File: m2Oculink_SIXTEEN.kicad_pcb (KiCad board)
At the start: 2 copper layers, 31.5 x 71.2 mm, 2 parts

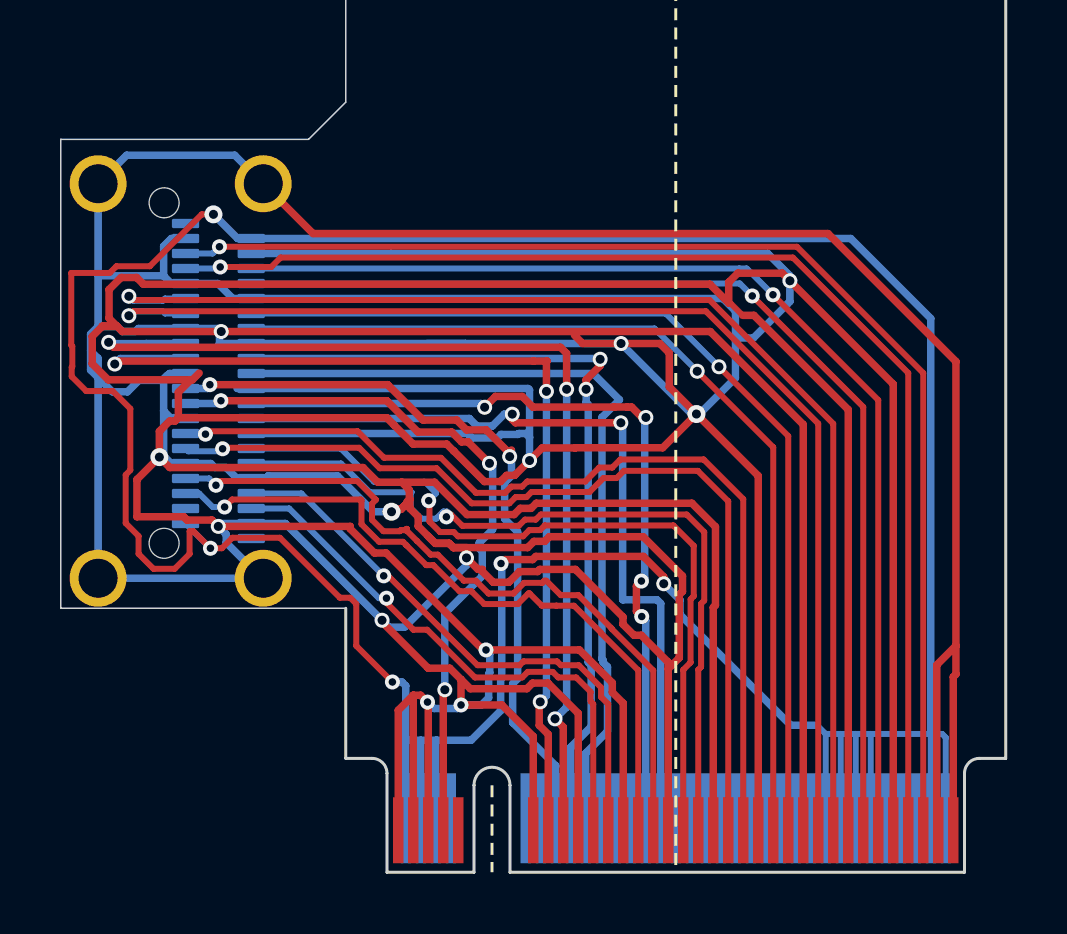
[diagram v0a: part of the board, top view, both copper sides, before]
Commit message: Update PCB
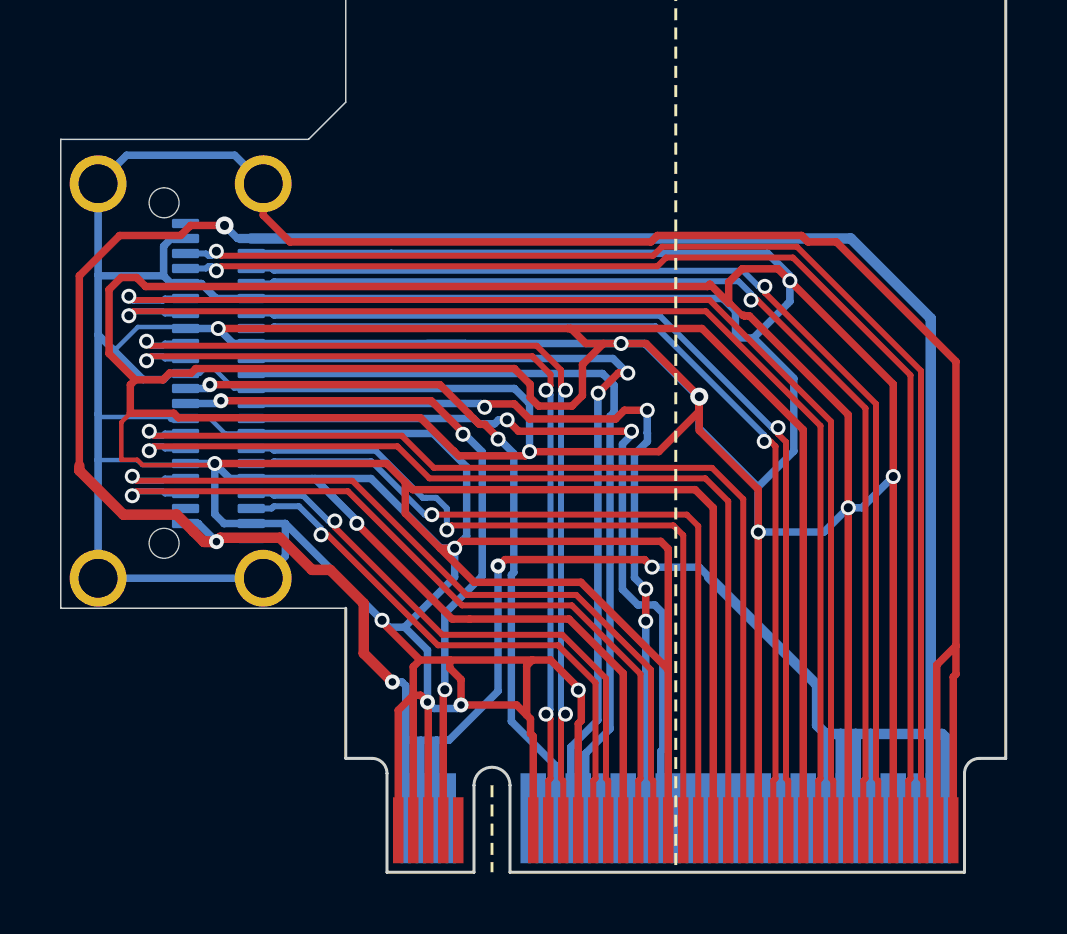
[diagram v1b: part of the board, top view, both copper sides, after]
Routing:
- net /GND: track 472.0 -> 503.1 mm, vias 13 -> 15
- net /3V3: track 122.9 -> 119.9 mm
- net /VCKN: track 34.2 -> 31.2 mm
- net /R0P: track 23.8 -> 26.6 mm
- net /R0N: track 24.7 -> 27.2 mm
- net /VCKP: track 32.8 -> 30.6 mm
- net /R1P: track 30.8 -> 32.4 mm
- net /R1N: track 31.5 -> 33.1 mm
- net /T1P: track 27.2 -> 26.0 mm
- net Net-(U1-CPRSNT/CLKREQ): track 27.5 -> 28.6 mm
- net /T1N: track 26.9 -> 26.0 mm
- net Net-(U1-CWAKE/PEWAKE): track 25.4 -> 24.8 mm
